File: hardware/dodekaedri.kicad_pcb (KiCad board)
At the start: 4 copper layers, 76.2 x 76.2 mm, 227 parts, among them CON401 BARREL_JACK, J801 HANDSFREE, P301 BNC, P801 TX_SW_WIRE, P802 USB_OTG, P803 UART, P804 PROG, P805 RNG_PINS, P806 CONN_01X08, P807 CONN_01X04, P808 CONN_02X04, P809 BOOT0JMPR, Q501 BCP56, Q502 IRL510, Q801 BSS84, SW801 SW_PUSH, SW802 SW, SW803 SW, SW804 SW, SW806 encoder, SW807 RESET, T301 TRANSFO, T302 TRANSFO, T501 TRANSFO2, T601 TRANSFO2, U201 MIC5365, U202 SI5351A, U401 NCP3170-D, U501 74LVC1G3157, U502 74LVC1G3157, U601 74LVC1G3157, U602 74LVC1G3157, U603 TL972IDR, U701 WM8731, U702 MCP6L02, U801 STM32F401, U802 WM8731

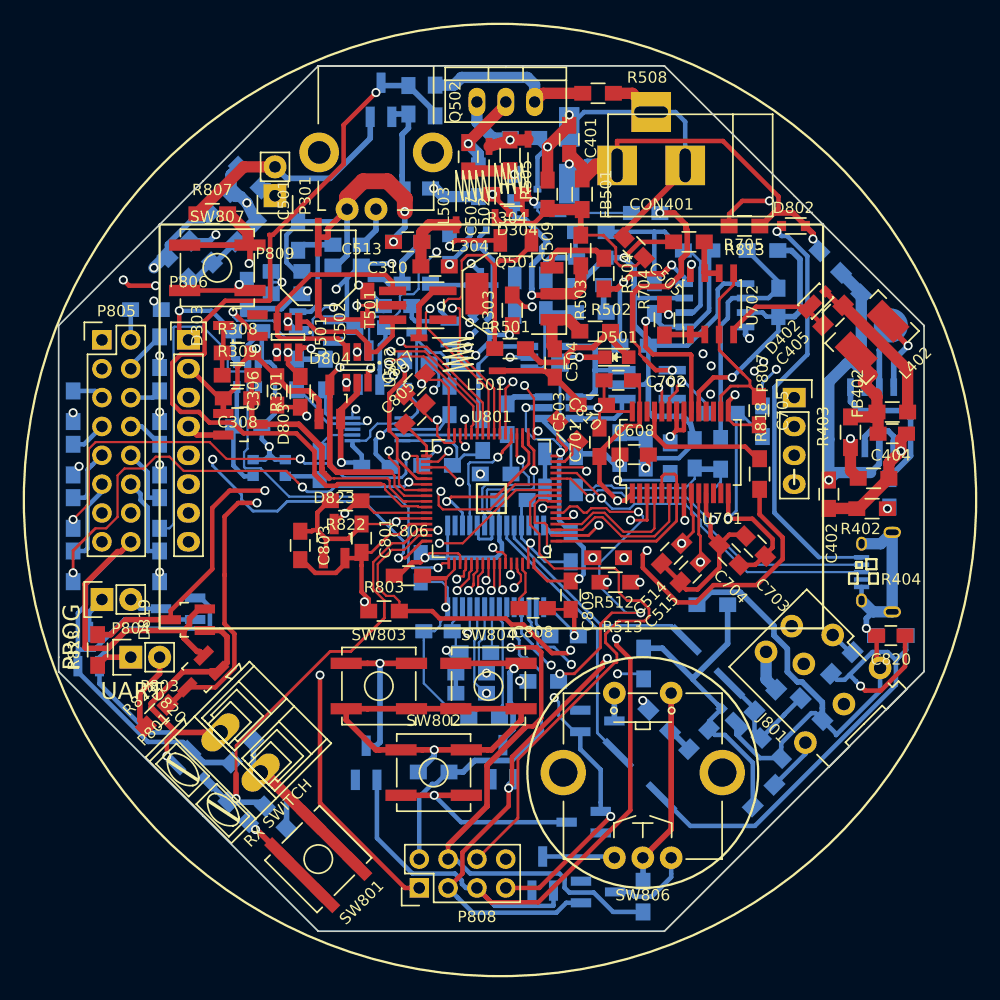
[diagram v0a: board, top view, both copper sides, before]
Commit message: layout done,d
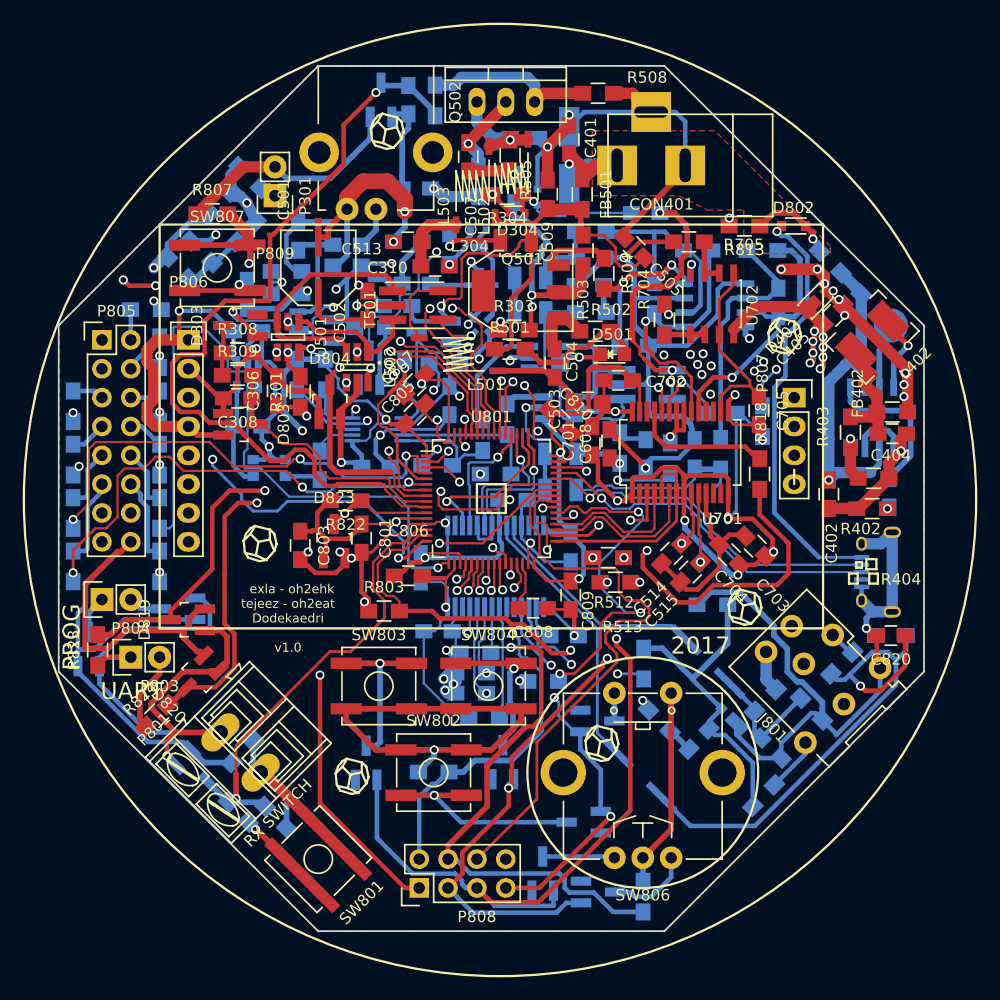
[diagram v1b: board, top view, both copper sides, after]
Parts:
- moved C608 2.36 mm to (153.9, 80.3), turned to 90 degrees
- moved R303 1.75 mm to (145.5, 70.3), turned to 0 degrees
- moved C810 1.17 mm to (149.5, 78.2)
- moved C701 0.65 mm to (152.4, 80.0)
- moved Q501 0.61 mm to (146.1, 66.8)
- moved D501 0.46 mm to (154.2, 72.4)
- moved C503 0.46 mm to (152.0, 76.6)
- moved R503 0.20 mm to (151.6, 63.2)
- moved R501 0.06 mm to (145.1, 71.9)
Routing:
- net +Vlogic: track 300.4 -> 407.5 mm, vias 16 -> 39
- net GND: track 440.7 -> 519.3 mm, vias 31 -> 43
- net Vin_net: track 41.4 -> 19.8 mm
- net /CPU/VIN_ADC: track 117.9 -> 113.6 mm
- net /CPU/RX_TX: track 26.8 -> 31.0 mm
- net /CPU/SWCLK: track 68.1 -> 71.6 mm
- net /RX_chain/RX_BIAS: track 56.4 -> 59.8 mm
- net Net-(R513-Pad1): track 31.5 -> 34.5 mm
- net Net-(D303-Pad2): track 39.3 -> 42.0 mm
- net Net-(L501-Pad1): track 5.49 -> 7.78 mm
- net /CPU/UI_SW_GRID1: track 103.6 -> 105.5 mm
- net /CPU/PB10: track 45.3 -> 46.8 mm
- net Net-(R818-Pad1): track 33.3 -> 34.8 mm
- net Net-(C306-Pad1): track 49.4 -> 48.0 mm
- net /CPU/UI_SW_GRID4: track 139.7 -> 141.0 mm
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- added copper zone on In1.Cu, net +Vlogic
- added copper zone on In2.Cu, net +Vlogic
- added copper zone on B.Cu, net GND
- added copper zone on F.Cu, net GND
- added copper zone on In1.Cu, net GND
- added copper zone on In2.Cu, net GND
- added copper zone on F.Cu, net Vin_net
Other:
- board text added: "2017"
- board text added: "exla - oh2ehk tejeez - oh2eat Dodekaedri v1.0"
- board text added: "oh2ti polyteknikkojen radiokerho r.y."
